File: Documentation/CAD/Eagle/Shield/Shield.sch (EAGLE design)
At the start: 26 parts, among them J2 KEYBOARD GROVE, M2 ARDUINO-PRO-MINI-3.3V, Q3 MOSFET-NCHANNEL2N7002PW

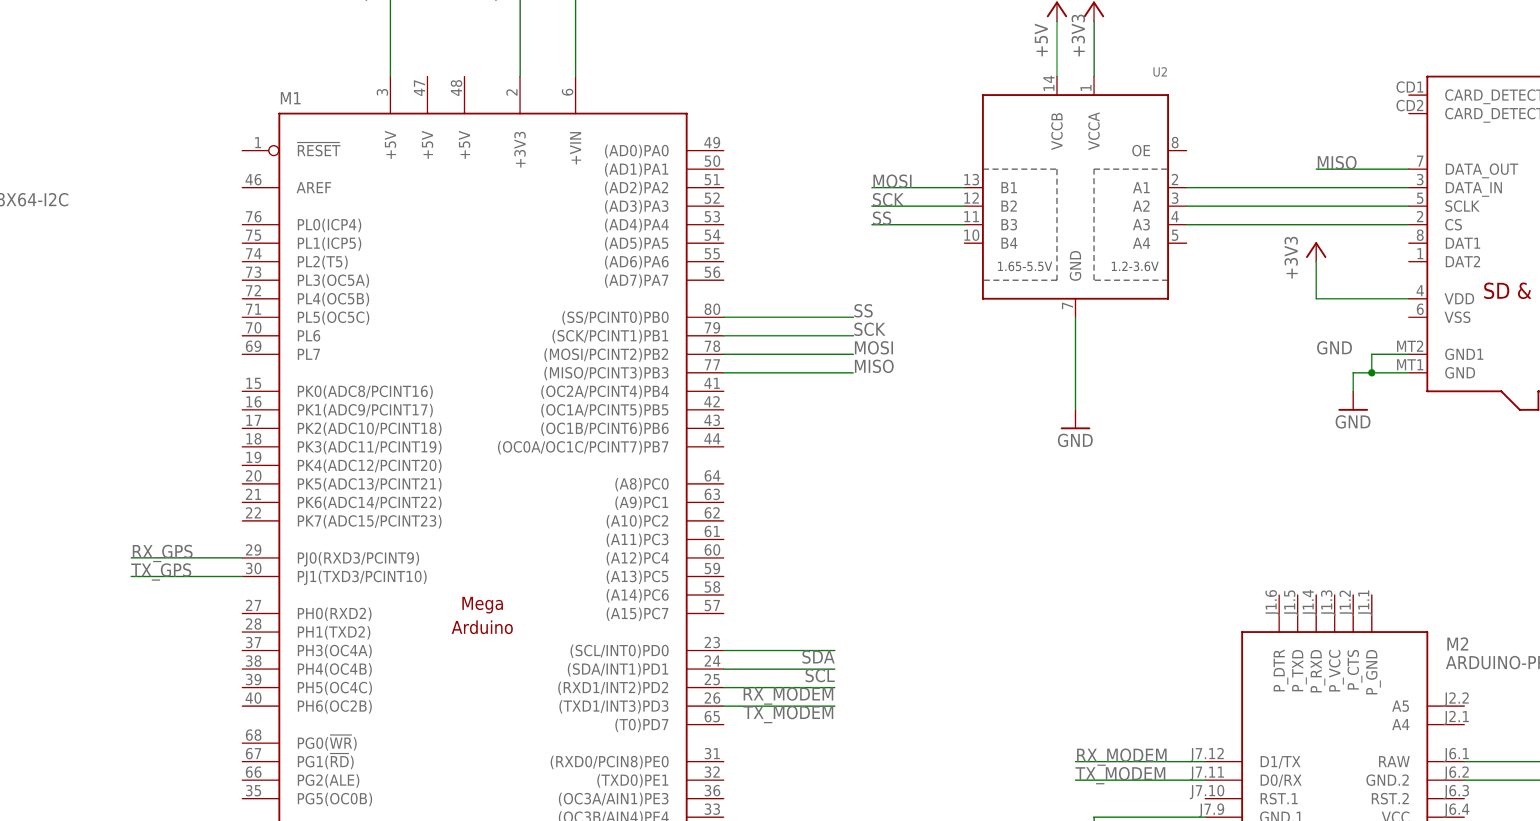
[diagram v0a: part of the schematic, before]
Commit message: Board fixes / improvements
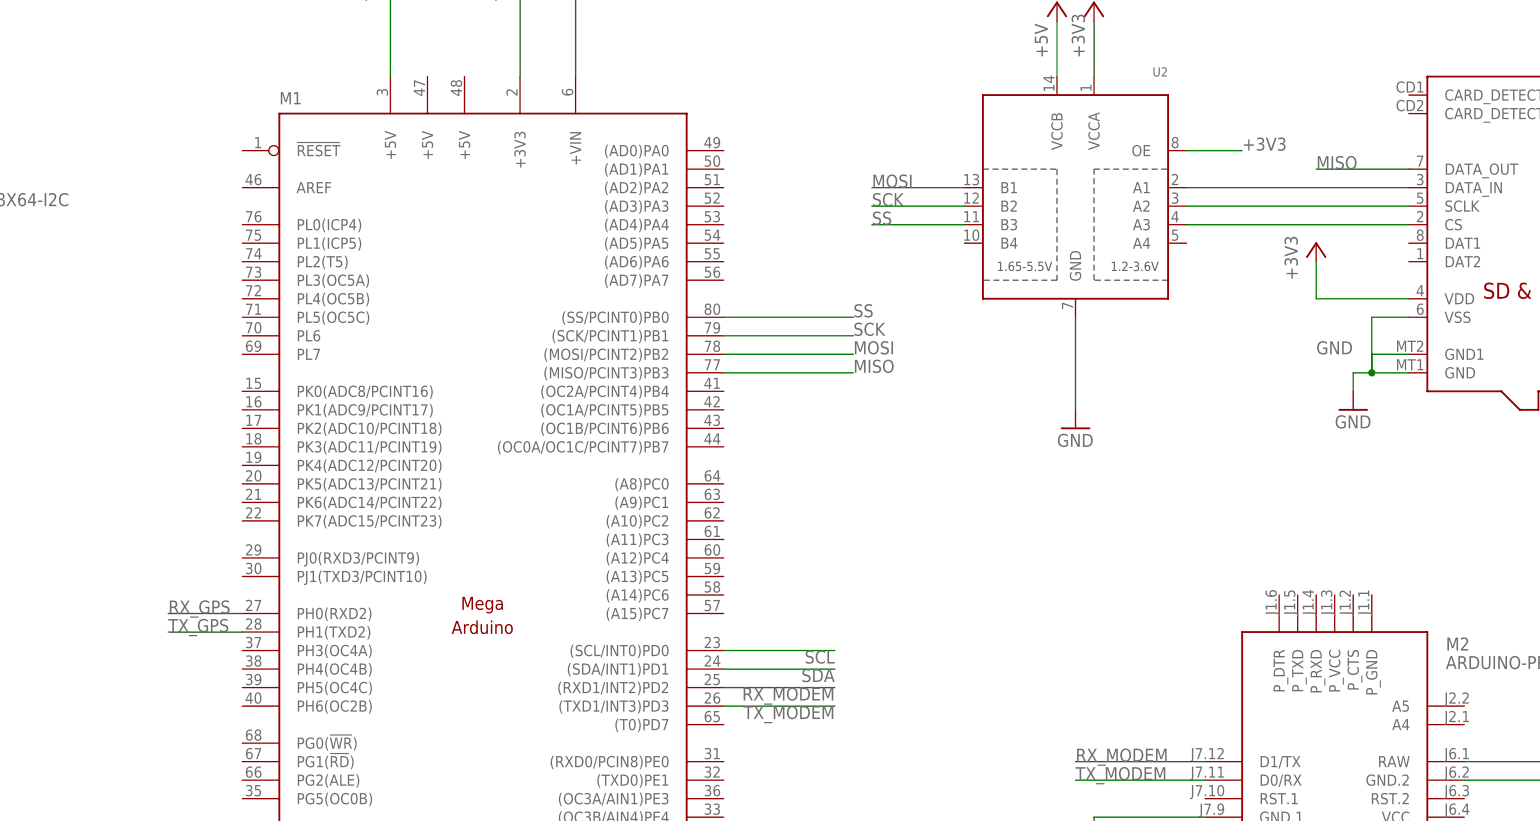
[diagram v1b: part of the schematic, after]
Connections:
- net +3V3: now also U2.OE
- net GND: now also SD.VSS
- net RX_GPS: now also M1.PH0(RXD2); no longer M1.PJ0(RXD3/PCINT9)
- net SCL: now also M1.(SCL/INT0)PD0; no longer M1.(SDA/INT1)PD1
- net SDA: now also M1.(SDA/INT1)PD1; no longer M1.(SCL/INT0)PD0
- net TX_GPS: now also M1.PH1(TXD2); no longer M1.PJ1(TXD3/PCINT10)
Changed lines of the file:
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@@
 <junction x="378.46" y="116.84"/>
 <label x="370.84" y="119.38" size="1.778" layer="95"/>
+<pinref part="SD" gate="G$1" pin="VSS"/>
+<wire x1="383.54" y1="124.46" x2="378.46" y2="124.46" width="0.1524" layer="91"/>
+<wire x1="378.46" y1="124.46" x2="378.46" y2="116.84" width="0.1524" layer="91"/>
 </segment>
 <segment>
@@
 </segment>
 <segment>
-<pinref part="M1" gate="G$1" pin="(SCL/INT0)PD0"/>
-<wire x1="289.56" y1="78.74" x2="304.8" y2="78.74" width="0.1524" layer="91"/>
-<label x="304.8" y="78.74" size="1.778" layer="95" rot="R180"/>
+<pinref part="M1" gate="G$1" pin="(SDA/INT1)PD1"/>
+<wire x1="289.56" y1="76.2" x2="304.8" y2="76.2" width="0.1524" layer="91"/>
+<label x="304.8" y="76.2" size="1.778" layer="95" rot="R180"/>
 </segment>
 </net>
@@
 </segment>
 <segment>
-<pinref part="M1" gate="G$1" pin="(SDA/INT1)PD1"/>
-<wire x1="289.56" y1="76.2" x2="304.8" y2="76.2" width="0.1524" layer="91"/>
-<label x="304.8" y="76.2" size="1.778" layer="95" rot="R180"/>
+<pinref part="M1" gate="G$1" pin="(SCL/INT0)PD0"/>
+<wire x1="289.56" y1="78.74" x2="304.8" y2="78.74" width="0.1524" layer="91"/>
+<label x="304.8" y="78.74" size="1.778" layer="95" rot="R180"/>
 </segment>
 </net>
@@
 <wire x1="370.84" y1="127" x2="370.84" y2="132.08" width="0.1524" layer="91"/>
 </segment>
+<segment>
+<pinref part="U2" gate="G$1" pin="OE"/>
+<wire x1="353.06" y1="147.32" x2="360.68" y2="147.32" width="0.1524" layer="91"/>
+<label x="360.68" y="147.32" size="1.778" layer="95"/>
+</segment>
 </net>
 <net name="N$3" class="0">
@@
 <net name="TX_GPS" class="0">
 <segment>
-<pinref part="M1" gate="G$1" pin="PJ1(TXD3/PCINT10)"/>
-<wire x1="223.52" y1="88.9" x2="208.28" y2="88.9" width="0.1524" layer="91"/>
-<label x="208.28" y="88.9" size="1.778" layer="95"/>
-</segment>
-<segment>
 <pinref part="GPS" gate="G$1" pin="RXD"/>
 <wire x1="25.4" y1="121.92" x2="15.24" y2="121.92" width="0.1524" layer="91"/>
 <label x="15.24" y="121.92" size="1.778" layer="95"/>
 </segment>
+<segment>
+<pinref part="M1" gate="G$1" pin="PH1(TXD2)"/>
+<wire x1="223.52" y1="81.28" x2="213.36" y2="81.28" width="0.1524" layer="91"/>
+<label x="213.36" y="81.28" size="1.778" layer="95"/>
+</segment>
 </net>
 <net name="RX_GPS" class="0">
-<segment>
-<pinref part="M1" gate="G$1" pin="PJ0(RXD3/PCINT9)"/>
-<wire x1="223.52" y1="91.44" x2="208.28" y2="91.44" width="0.1524" layer="91"/>
-<label x="208.28" y="91.44" size="1.778" layer="95"/>
-</segment>
 <segment>
 <pinref part="GPS" gate="G$1" pin="TXD"/>
@@
 <label x="15.24" y="124.46" size="1.778" layer="95"/>
 </segment>
-</net>
+<segment>
+<pinref part="M1" gate="G$1" pin="PH0(RXD2)"/>
+<wire x1="223.52" y1="83.82" x2="213.36" y2="83.82" width="0.1524" layer="91"/>
+<label x="213.36" y="83.82" size="1.778" layer="95"/>
+</segment>
+</net>
